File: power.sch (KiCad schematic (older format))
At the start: 37 parts, among them Q1 Q_PMOS_GSD, SW1 Power switch, U1 SY8079AAC, U2 SY8079AAC, U3 XT4054K421MR-G, U4 SY6280AAC, U5 SY6280AAC

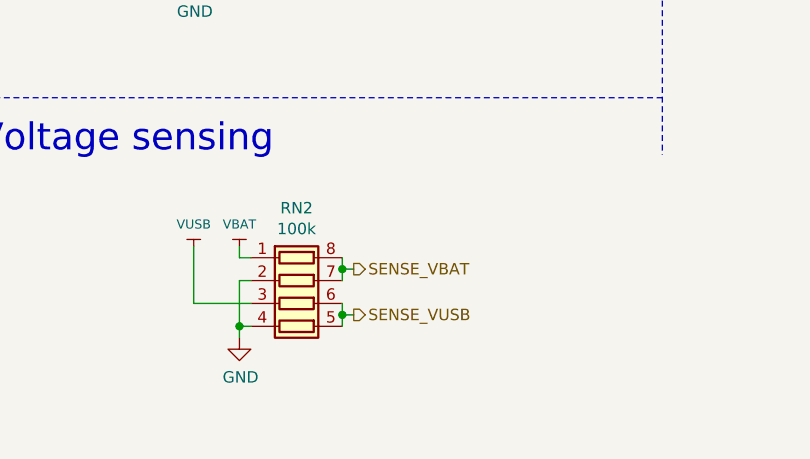
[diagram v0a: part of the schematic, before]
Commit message: Dump.
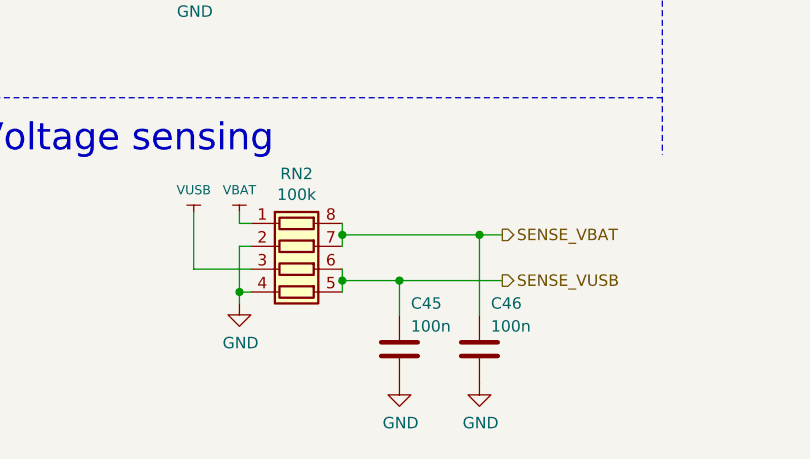
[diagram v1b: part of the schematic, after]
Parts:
- added C45, C46: 100n, Capacitor_SMD:C_0603_1608Metric, symbol Device:C
- BT1: Price 0.12 -> (none)
- C10, C11, C12, C15, C4, C5, C9: footprint Capacitor_SMD:C_0603_1608Metric -> Capacitor_SMD:C_0805_2012Metric; LCSC (none) -> C5674; Price 0.0020 -> (none)
- C13, C3: LCSC (none) -> C307461; Price 0.0020 -> (none)
- C14, C6: Price 0.0020 -> (none)
- C7, C8: LCSC (none) -> C388041; Price 0.0020 -> (none)
- D2: LCSC (none) -> C232573; Sponsored (none) -> N
- D3: LCSC - -> C383224; Price 0.053 -> (none)
- L1, L2: Price 0.026 -> (none)
- Q1: LCSC (none) -> C180952; Sponsored (none) -> N
- R10, R4, R7: LCSC - -> C269690; Price 0.0005 -> (none)
- R11, R12, R13, R5, R6, R9: LCSC - -> C115324; Price 0.0005 -> (none)
- R14: Price 0.0016 -> (none)
- R8: LCSC - -> C23058; Price 0.0005 -> (none)
- RN2: Price 0.0042 -> (none)
- SW1: Price 0.023 -> (none)
- U1, U2: Price 0.067 -> (none)
- U3: Price 0.028 -> (none)
- U4, U5: Price 0.061 -> (none)
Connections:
- net GND: now also C45.2, C46.2
- net SENSE_VBAT: now also C46.1
- net SENSE_VUSB: now also C45.1
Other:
- moved on the sheet: RN2

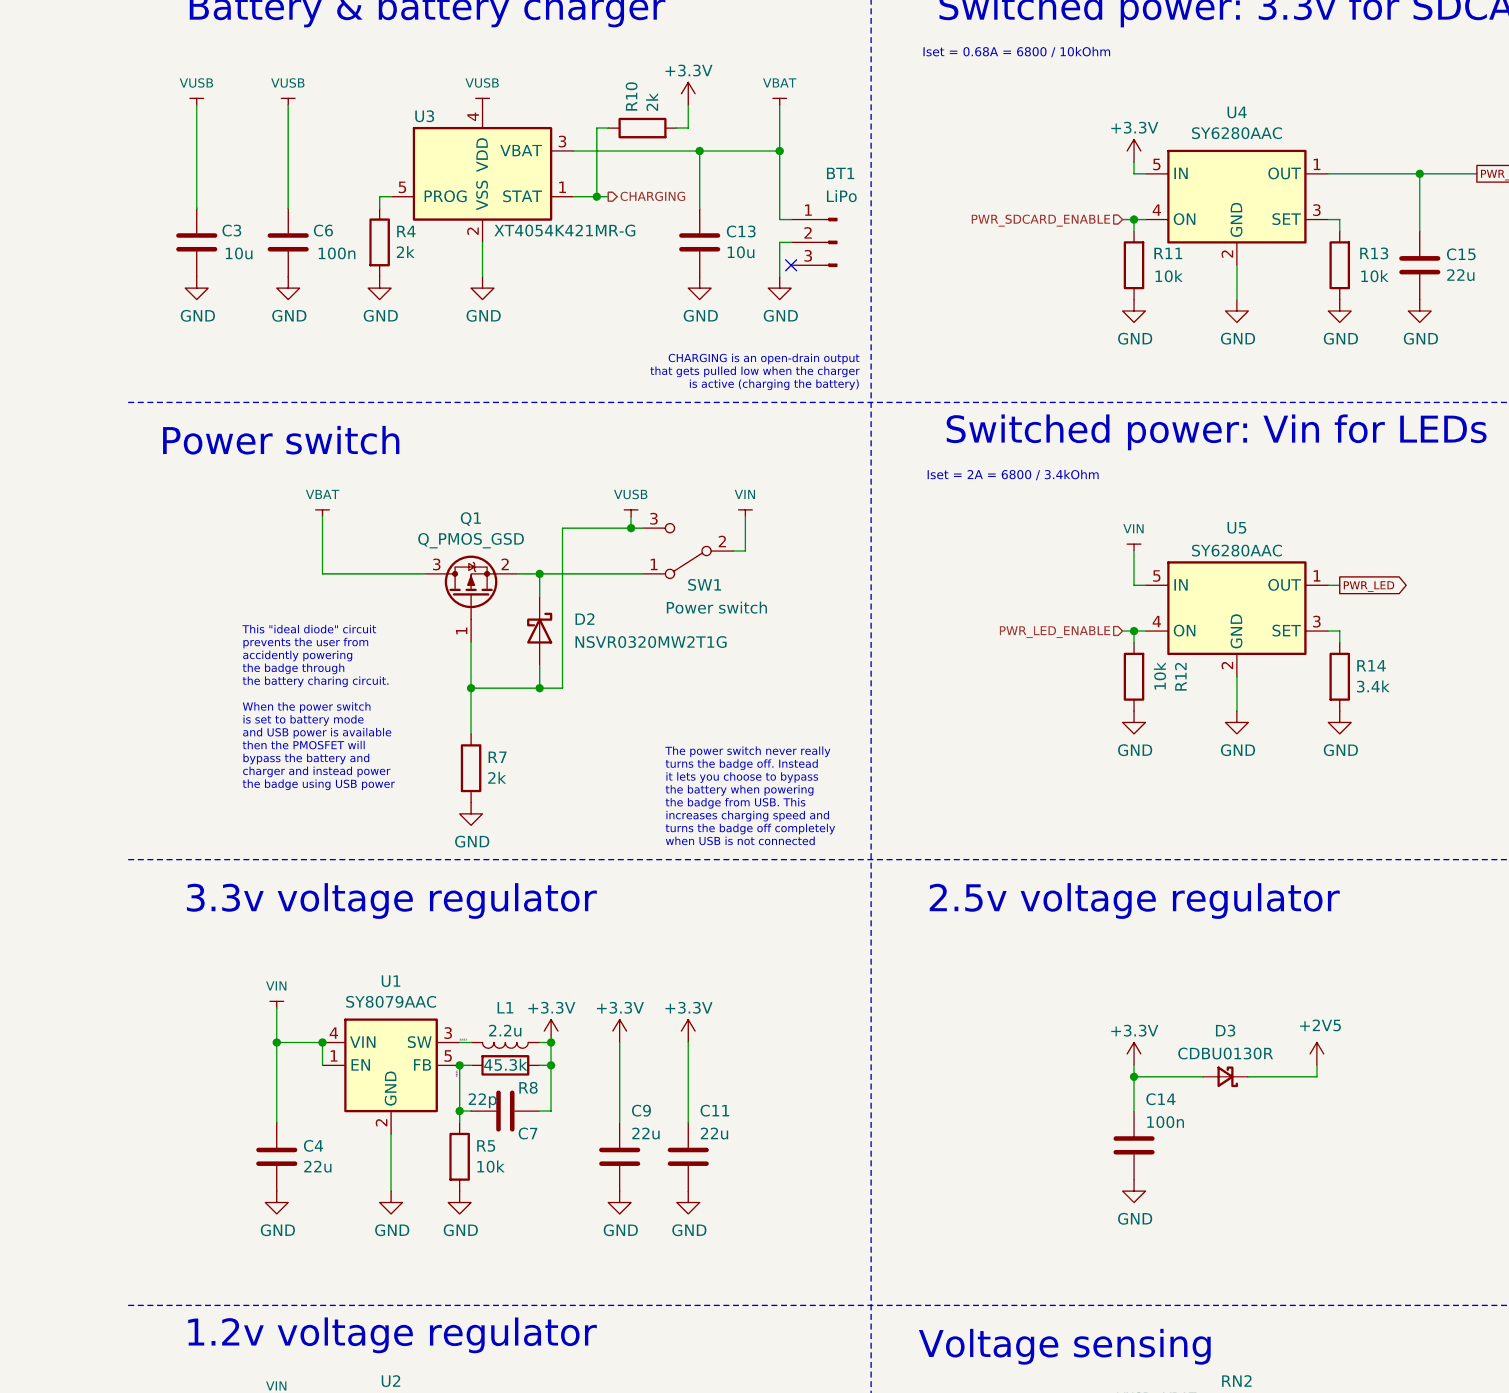
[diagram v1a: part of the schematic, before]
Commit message: Work in progress: prototype 2
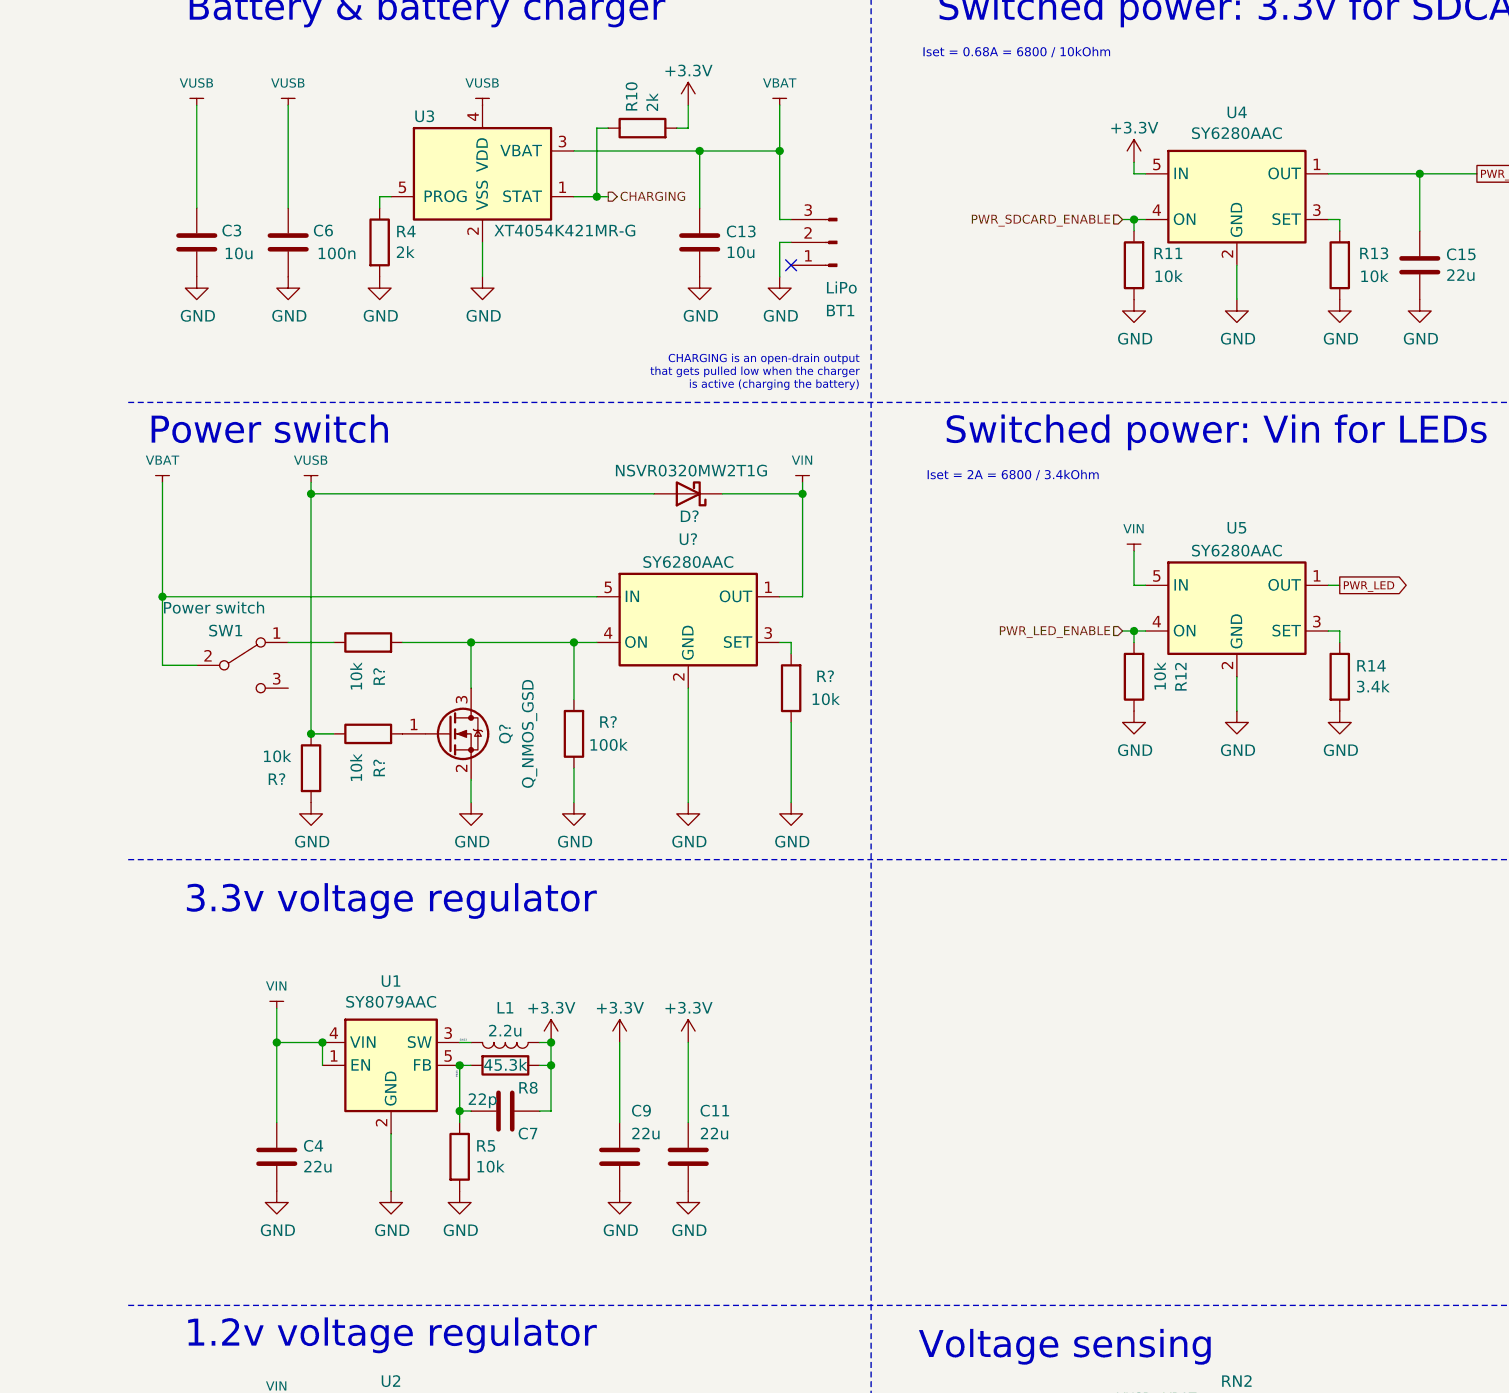
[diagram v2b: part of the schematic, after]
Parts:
- removed C14: 100n, Capacitor_SMD:C_0603_1608Metric, symbol Device:C
- removed D2: NSVR0320MW2T1G, Diode_SMD:D_SOD-323, symbol Device:D_Schottky
- removed D3: CDBU0130R, Diode_SMD:D_0603_1608Metric, symbol Device:D_Schottky_Small
- removed Q1: Q_PMOS_GSD, Package_TO_SOT_SMD:SOT-23, symbol Device:Q_PMOS_GSD
- removed R7: 2k, Resistor_SMD:R_0603_1608Metric, symbol Device:R
- added D?: NSVR0320MW2T1G, Diode_SMD:D_SOD-323, symbol Device:D_Schottky
- added Q?: Q_NMOS_GSD, Package_TO_SOT_SMD:SOT-23, symbol Device:Q_NMOS_GSD
- added R? (x4): 10k, Resistor_SMD:R_0603_1608Metric, symbol Device:R
- added R?: 100k, Resistor_SMD:R_0603_1608Metric, symbol Device:R
- added U?: SY6280AAC, Package_TO_SOT_SMD:SOT-23-5, symbol Power_Management:AAT4610BIGV-1-T1
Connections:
- net GND: now also Q?.2 (S), R?.1, R?.1, R?.2, U?.2 (GND)
- net VBAT: now also BT1.3 (Pin_3), SW1.2 (B), U?.5 (IN); no longer BT1.1 (Pin_1)
- net VIN: now also D?.1 (K), U?.1 (OUT); no longer SW1.2 (B)
- net VUSB: now also D?.2 (A), R?.1, R?.1; no longer SW1.3 (C)
- net at SW1.1 (A): now also R?.1
- new net: R?.2, U?.3 (SET)
- new net: Q?.3 (D), R?.2, R?.2, U?.4 (ON)
- new net: Q?.1 (G), R?.2
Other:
- note removed: "2.5v voltage regulator"
- note removed: "The power switch never really\nturns the badge off. Instead\nit lets you choose to bypass\nthe battery when powering\nthe badge from USB. This\nincreases charging speed and\nturns the badge off completely\nwhen USB is not connected"
- note removed: "This "ideal diode" circuit\nprevents the user from\naccidently powering\nthe badge through\nthe battery charing circuit.\n\nWhen the power switch\nis set to battery mode\nand USB power is available\nthen the PMOSFET will\nbypass the battery and\ncharger and instead power\nthe badge using USB power"
- moved on the sheet: SW1
